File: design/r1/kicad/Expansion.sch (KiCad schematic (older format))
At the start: 12 parts, among them IC7 7404N, IC9 74LS01N, J5 GPIO-PANEL

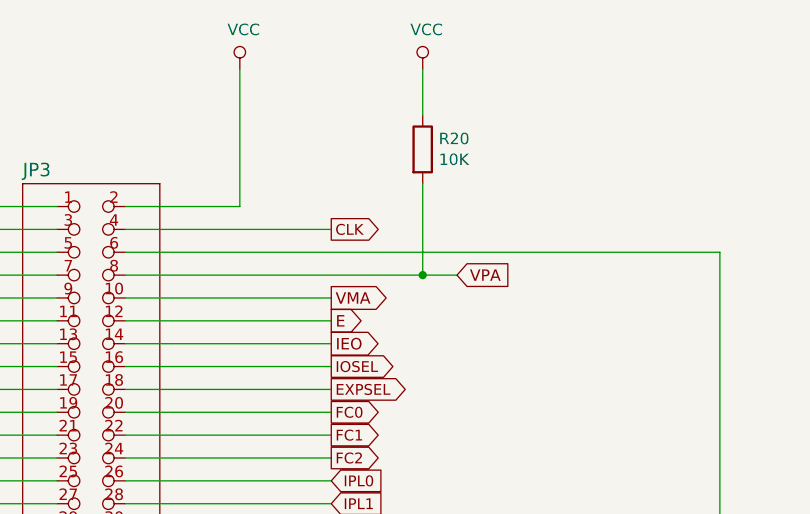
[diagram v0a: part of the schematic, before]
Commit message: Design complete
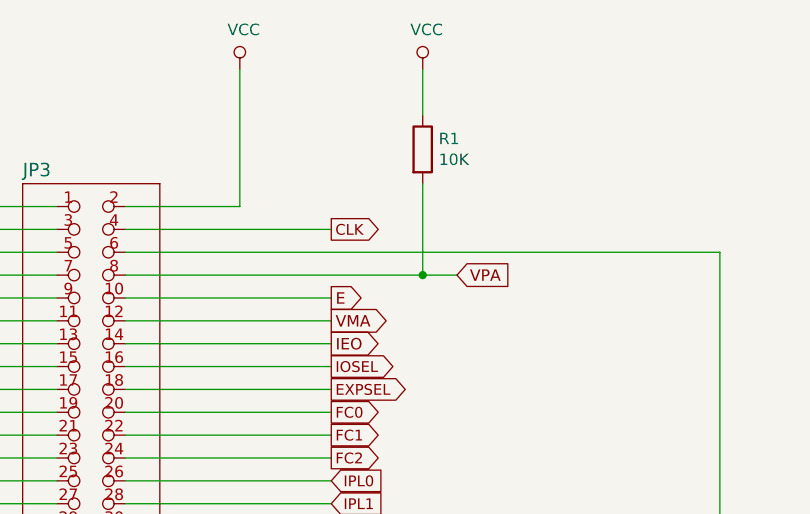
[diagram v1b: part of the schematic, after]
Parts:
- J5: footprint (none) -> Connector_PinHeader_2.54mm:PinHeader_2x08_P2.54mm_Vertical
- R1: renamed from R20; footprint (none) -> rosco_m68k:0207_10
- R18, R19: footprint (none) -> rosco_m68k:0207_10
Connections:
- net E: now also JP3.10; no longer JP3.12
- net VMA: now also JP3.12; no longer JP3.10
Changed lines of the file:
@@
 F 0 "J5" H 15300 5217 50  0000 C CNN
 F 1 "GPIO-PANEL" H 15300 5126 50  0000 C CNN
-F 2 "" H 15250 4700 50  0001 C CNN
+F 2 "Connector_PinHeader_2.54mm:PinHeader_2x08_P2.54mm_Vertical" H 15250 4700 50  0001 C CNN
 F 3 "~" H 15250 4700 50  0001 C CNN
 	1    15250 4700
@@
 Text GLabel 10450 3700 2    50   Input ~ 0
 VPA
+Text GLabel 9900 3900 2    50   Output ~ 0
+VMA
 Text GLabel 9900 3800 2    50   Output ~ 0
-VMA
-Text GLabel 9900 3900 2    50   Output ~ 0
 E
 $Comp
@@
 F 0 "R18" H 14870 5496 50  0000 L CNN
 F 1 "4K7" H 14870 5405 50  0000 L CNN
-F 2 "" V 14730 5450 50  0001 C CNN
+F 2 "rosco_m68k:0207_10" V 14730 5450 50  0001 C CNN
 F 3 "~" H 14800 5450 50  0001 C CNN
 	1    14800 5450
@@
 F 0 "R19" H 15870 5496 50  0000 L CNN
 F 1 "4K7" H 15870 5405 50  0000 L CNN
-F 2 "" V 15730 5450 50  0001 C CNN
+F 2 "rosco_m68k:0207_10" V 15730 5450 50  0001 C CNN
 F 3 "~" H 15800 5450 50  0001 C CNN
 	1    15800 5450
@@
 	15300 5850 15800 5850
 $Comp
-L Device:R R20
+L Device:R R1
 U 1 1 600B8632
 P 10300 3150
-F 0 "R20" H 10370 3196 50  0000 L CNN
+F 0 "R1" H 10370 3196 50  0000 L CNN
 F 1 "10K" H 10370 3105 50  0000 L CNN
-F 2 "" V 10230 3150 50  0001 C CNN
+F 2 "rosco_m68k:0207_10" V 10230 3150 50  0001 C CNN
 F 3 "~" H 10300 3150 50  0001 C CNN
 	1    10300 3150
@@
 Wire Wire Line
 	14800 5100 14350 5100
+Text GLabel 16150 4800 2    50   Output ~ 0
+IOSEL
+Text GLabel 16150 4900 2    50   Output ~ 0
+EXPSEL
 Wire Bus Line
 	8000 6900 8000 7200
@@
 Wire Bus Line
 	7500 3050 7500 5400
-Text GLabel 16150 4800 2    50   Output ~ 0
-IOSEL
-Text GLabel 16150 4900 2    50   Output ~ 0
-EXPSEL
 $EndSCHEMATC
